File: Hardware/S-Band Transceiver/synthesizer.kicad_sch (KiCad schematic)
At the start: 1 part, among them U10 ADF4351

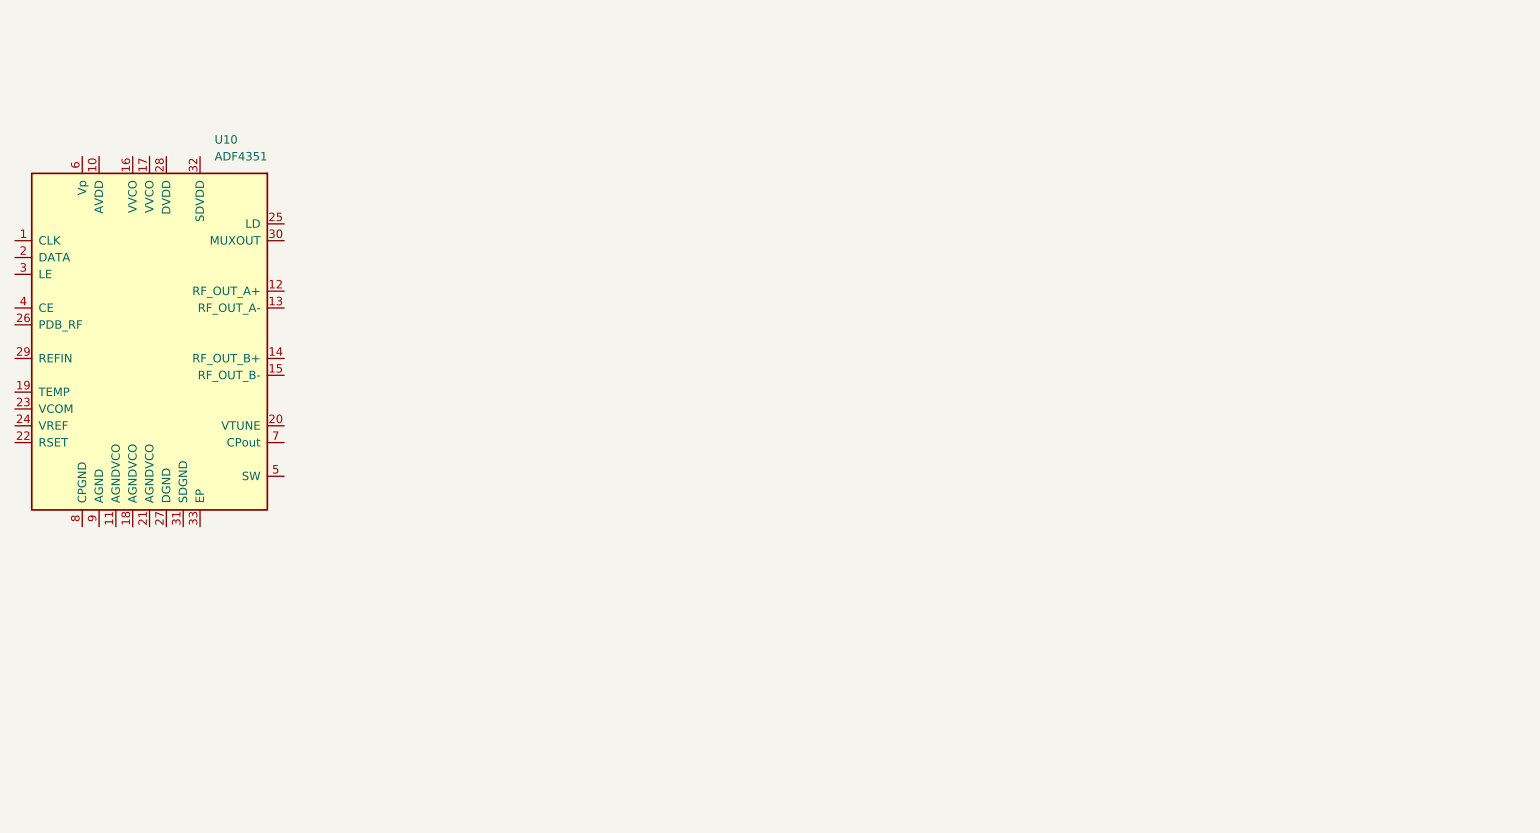
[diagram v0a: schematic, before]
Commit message: Working on schematic for adf4351
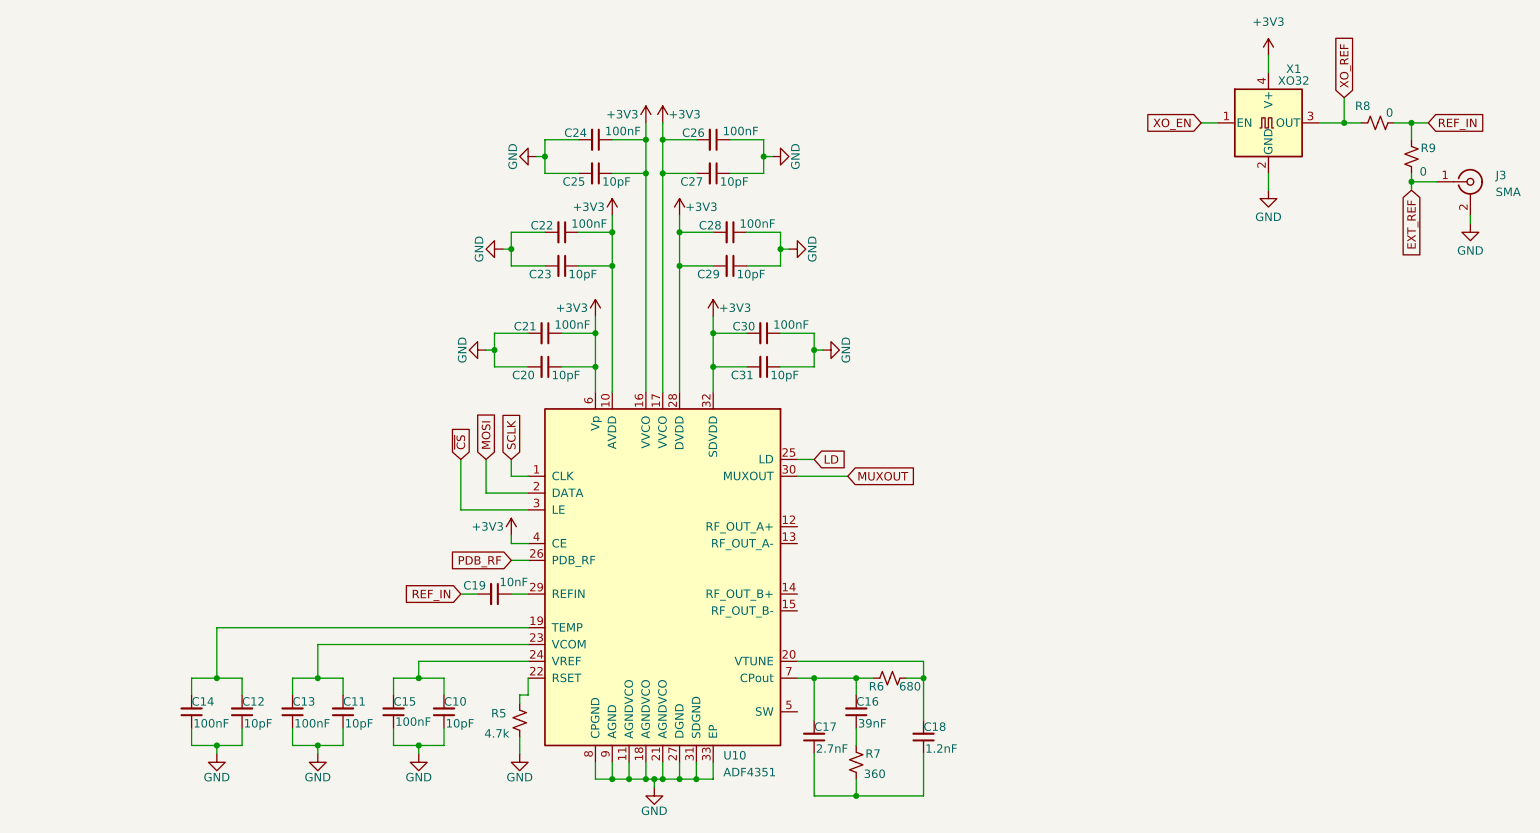
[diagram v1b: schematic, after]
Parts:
- added C10, C11, C12, C20, C23, C25, C27, C29, C31: 10pF, symbol Device:C_Small
- added C13, C14, C15, C21, C22, C24, C26, C28, C30: 100nF, symbol Device:C_Small
- added C16: 39nF, symbol Device:C_Small
- added C17: 2.7nF, symbol Device:C_Small
- added C18: 1.2nF, symbol Device:C_Small
- added C19: 10nF, symbol Device:C_Small
- added J3: SMA, symbol Connector:Conn_Coaxial
- added R5: 4.7k, symbol Device:R_Small_US
- added R6: 680, symbol Device:R_Small_US
- added R7: 360, symbol Device:R_Small_US
- added R8, R9: 0, symbol Device:R_Small_US
- added X1: XO32, Oscillator:Oscillator_SMD_EuroQuartz_XO91-4Pin_7.0x5.0mm, symbol Oscillator:XO32
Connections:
- net SCLK: now reaches U10.1 (CLK)
- net +3V3: now reaches U10.10 (AVDD)
- net +3V3: now also U10.16 (VVCO), U10.17 (VVCO), U10.28 (DVDD), U10.32 (SDVDD), U10.4 (CE), U10.6 (Vp), C20.1, C21.1, C22.1, C23.1, C24.1, C25.1, C26.2, C27.2, C28.2, C29.2, C30.2, C31.2, X1.4 (V+)
- net GND: now reaches U10.11 (AGNDVCO)
- net GND: now also U10.18 (AGNDVCO), U10.21 (AGNDVCO), U10.27 (DGND), U10.31 (SDGND), U10.33 (EP), U10.8 (CPGND), U10.9 (AGND), C10.1, C11.1, C12.1, C13.1, C14.1, C15.1, C20.2, C21.2, C22.2, C23.2, C24.2, C25.2, C26.1, C27.1, C28.1, C29.1, C30.1, C31.1, J3.2 (Ext), R5.2, X1.2 (GND)
- net at U10.19 (TEMP): now also C12.2, C14.2
- net MOSI: now reaches U10.2 (DATA)
- net at U10.20 (VTUNE): now also C18.2, R6.2
- net at U10.22 (RSET): now also R5.1
- net at U10.23 (VCOM): now also C11.2, C13.2
- net at U10.24 (VREF): now also C10.2, C15.2
- net LD: now reaches U10.25 (LD)
- net PDB_RF: now reaches U10.26 (PDB_RF)
- net at U10.29 (REFIN): now also C19.1
- net ~{CS}: now reaches U10.3 (LE)
- net MUXOUT: now reaches U10.30 (MUXOUT)
- net at U10.7 (CPout): now also C16.2, C17.2, R6.1
- new net: C17.1, C18.1, R7.1
- new net: C16.1, R7.2
- new net EXT_REF: J3.1 (In), R9.1
- new net REF_IN: C19.2, R8.2, R9.2
- new net XO_EN: X1.1 (EN)
- new net XO_REF: R8.1, X1.3 (OUT)
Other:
- moved on the sheet: U10
